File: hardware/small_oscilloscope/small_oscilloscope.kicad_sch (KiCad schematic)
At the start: 8 parts, among them J2 Parellel LCD, J5 Conn_01x16, J6 Conn_01x16, Q9 NTR5103NT1G, U2 FT800Q-T, Y1 12.0000M

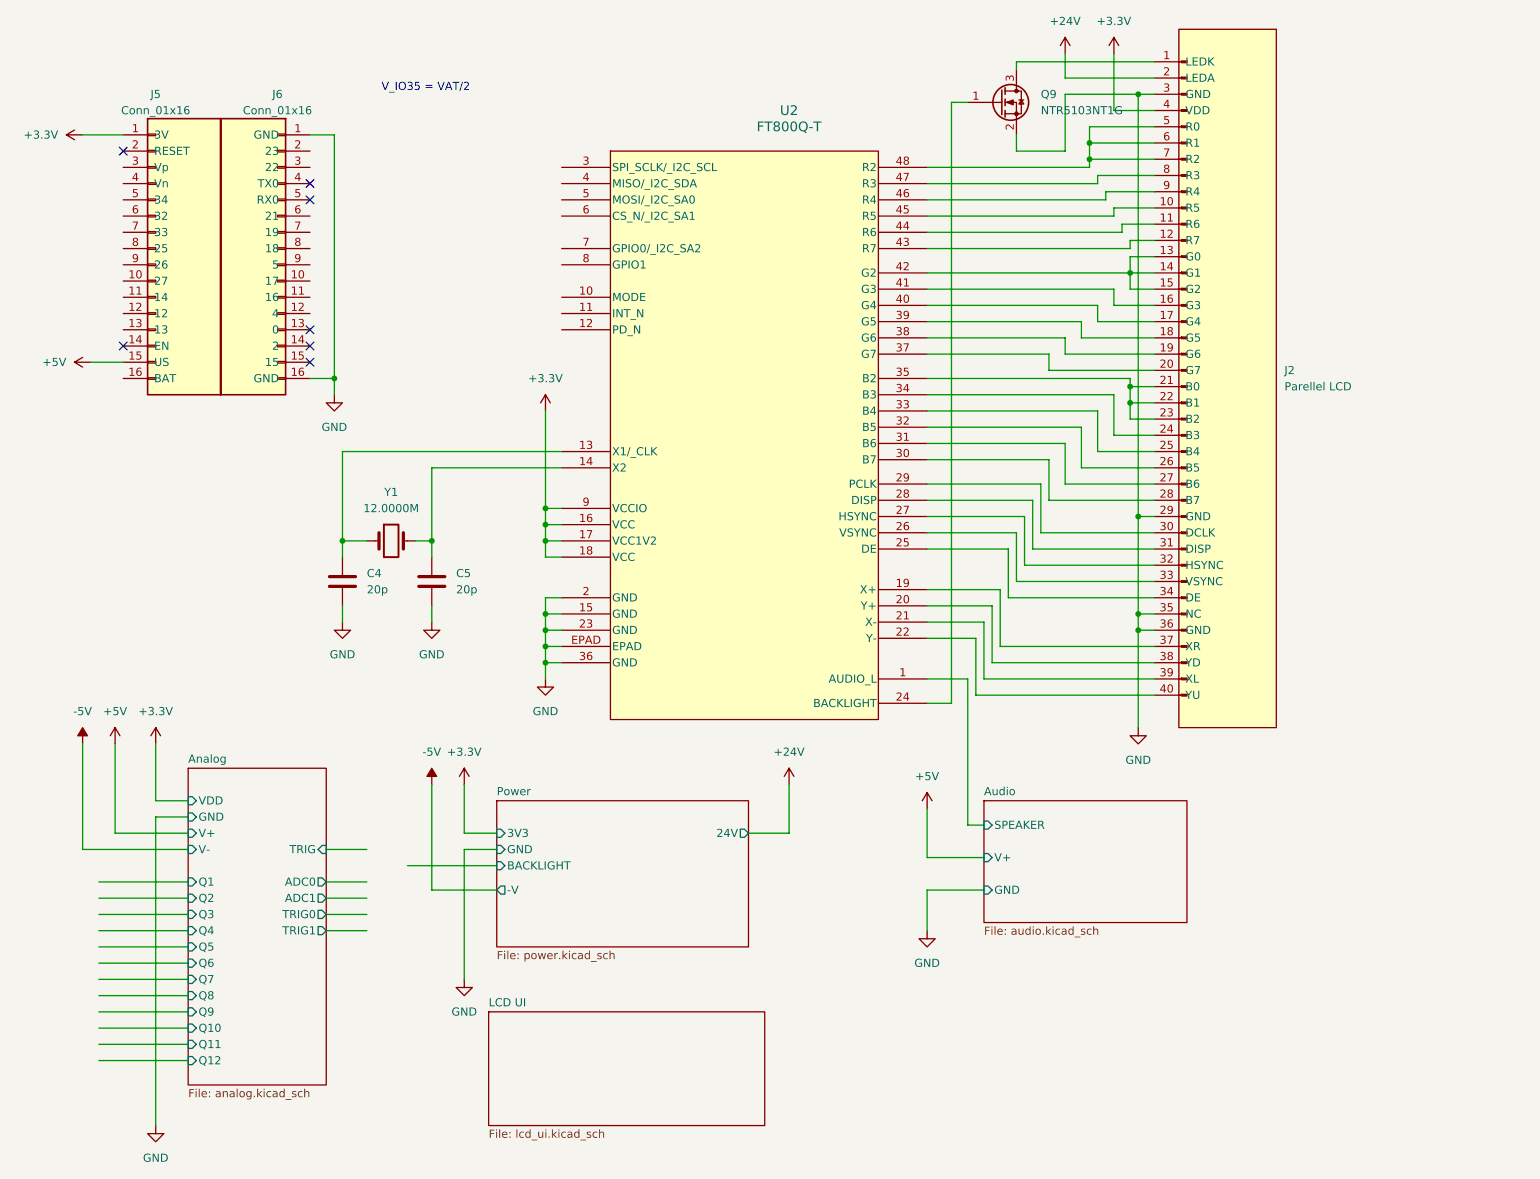
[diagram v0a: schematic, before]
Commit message: 250627 circuit
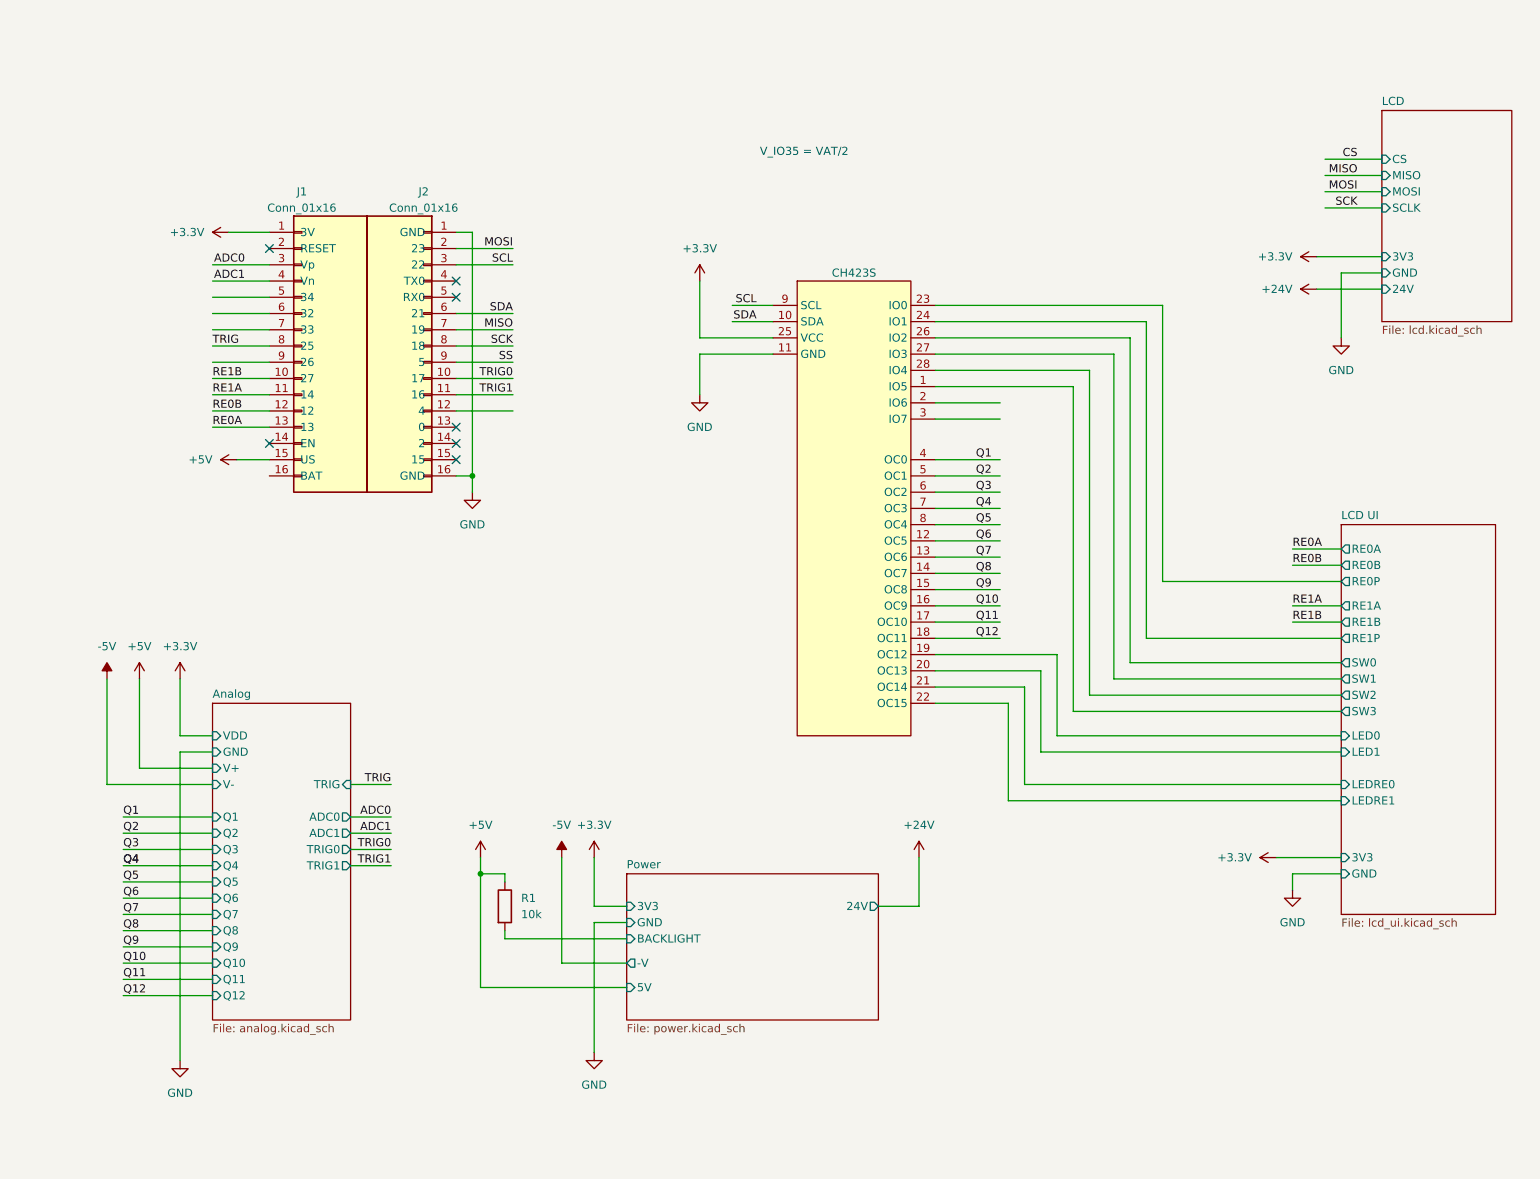
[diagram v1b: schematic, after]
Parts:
- removed C4, C5: 20p, Capacitor_THT:C_Disc_D3.8mm_W2.6mm_P2.50mm, symbol Device:C
- removed J2: Parellel LCD, Connector_FFC-FPC:TE_4-1734839-0_1x40-1MP_P0.5mm_Horizontal, symbol LCD_interface:Conn_01x40_Pin
- removed Q9: NTR5103NT1G, symbol Transistor_FET:Q_NMOS_GSD
- removed U2: FT800Q-T, VQFN48_FT800_BRI, symbol FT800:FT800Q-T
- removed Y1: 12.0000M, Crystal:Crystal_HC49-4H_Vertical, symbol Device:Crystal
- added R1: 10k, Resistor_SMD:R_0402_1005Metric_Pad0.72x0.64mm_HandSolder, symbol Device:R
- added U1: CH423S, Package_SO:SOP-28_8.4x18.16mm_P1.27mm, symbol giho_user:CH423s
- renumbered J5 to J1, J6 to J2
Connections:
- net +3.3V: now also U1.25 (VCC)
- net +5V: now also R1.1
- net GND: now also U1.11 (GND)
- net Power/BACKLIGHT: now also R1.2
- net TRIG0: now reaches J2.10 (17)
- net TRIG1: now reaches J2.11 (16)
- net MOSI: now reaches J2.2 (23)
- net SCL: now reaches J2.3 (22)
- net SCL: now also U1.9 (SCL)
- net SDA: now reaches J2.6 (21)
- net SDA: now also U1.10 (SDA)
- net MISO: now reaches J2.7 (19)
- net SCK: now reaches J2.8 (18)
- net SS: now reaches J2.9 (5)
- net RE1B: now reaches J1.10 (27)
- net RE1A: now reaches J1.11 (14)
- net RE0B: now reaches J1.12
- net RE0A: now reaches J1.13
- net ADC0: now reaches J1.3 (Vp)
- net ADC1: now reaches J1.4 (Vn)
- net TRIG: now reaches J1.8 (25)
- new net LCD UI/LED0: U1.19 (OC12)
- new net LCD UI/LED1: U1.20 (OC13)
- new net LCD UI/LEDRE0: U1.21 (OC14)
- new net LCD UI/LEDRE1: U1.22 (OC15)
- new net LCD UI/RE0P: U1.23 (IO0)
- new net LCD UI/RE1P: U1.24 (IO1)
- new net LCD UI/SW0: U1.26 (IO2)
- new net LCD UI/SW1: U1.27 (IO3)
- new net LCD UI/SW2: U1.28 (IO4)
- new net LCD UI/SW3: U1.1 (IO5)
- new net Q1: U1.4 (OC0)
- new net Q10: U1.16 (OC9)
- new net Q11: U1.17 (OC10)
- new net Q12: U1.18 (OC11)
- new net Q2: U1.5 (OC1)
- new net Q3: U1.6 (OC2)
- new net Q4: U1.7 (OC3)
- new net Q5: U1.8 (OC4)
- new net Q6: U1.12 (OC5)
- new net Q7: U1.13 (OC6)
- new net Q8: U1.14 (OC7)
- new net Q9: U1.15 (OC8)
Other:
- removed sheet Audio
- added sheet LCD (lcd.kicad_sch)
- sheet LCD UI ports: added 3V3, GND, LED0, LED1, LEDRE0, LEDRE1, RE0A, RE0B, RE0P, RE1A, RE1B, RE1P, SW0, SW1, SW2, SW3; removed none
- sheet Power ports: added 5V; removed none
- moved on the sheet: J1, J2
